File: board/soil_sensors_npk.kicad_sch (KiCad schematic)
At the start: 7 parts, among them J2 Conn_01x04_MountingPin, U6 MAX3485

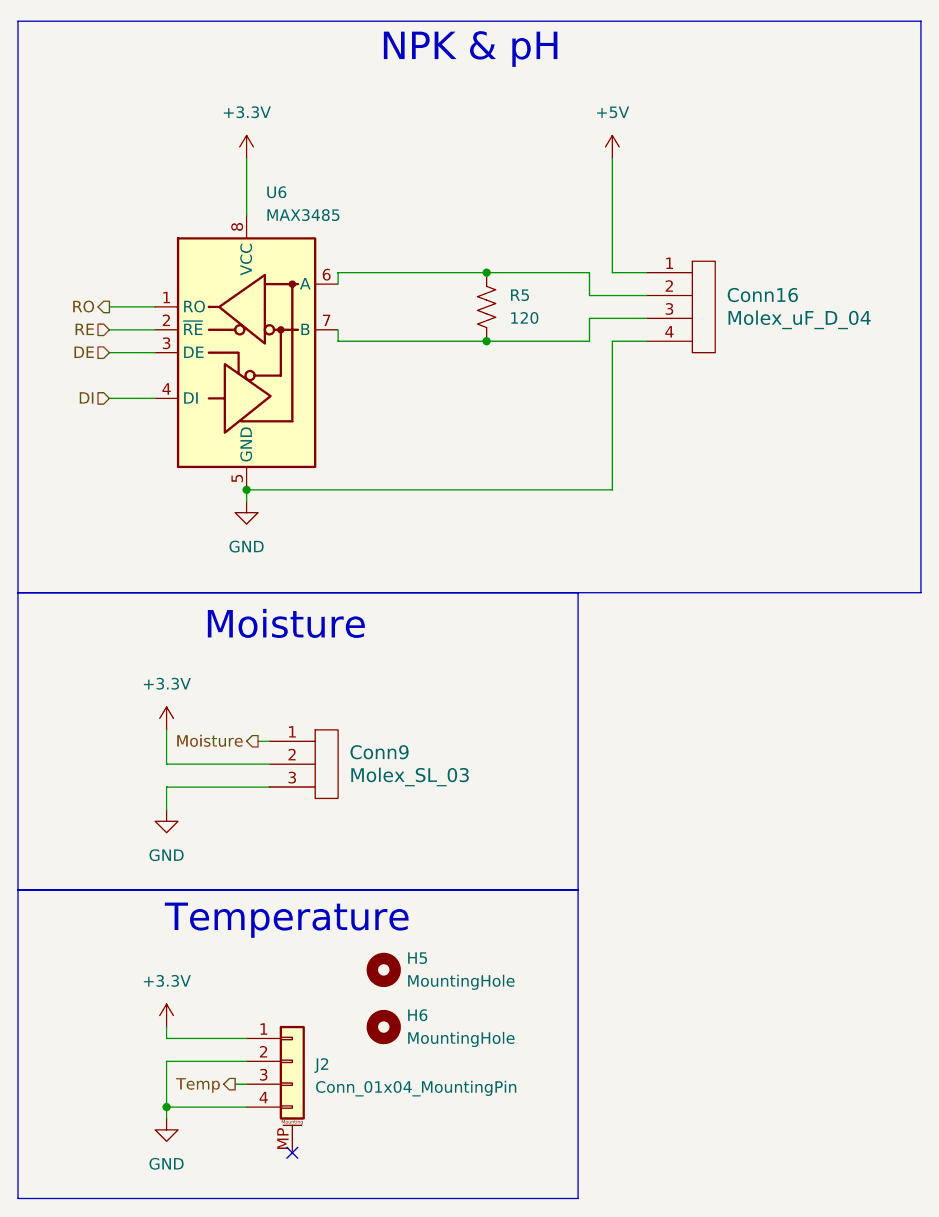
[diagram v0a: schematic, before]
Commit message: Redesigning Layout
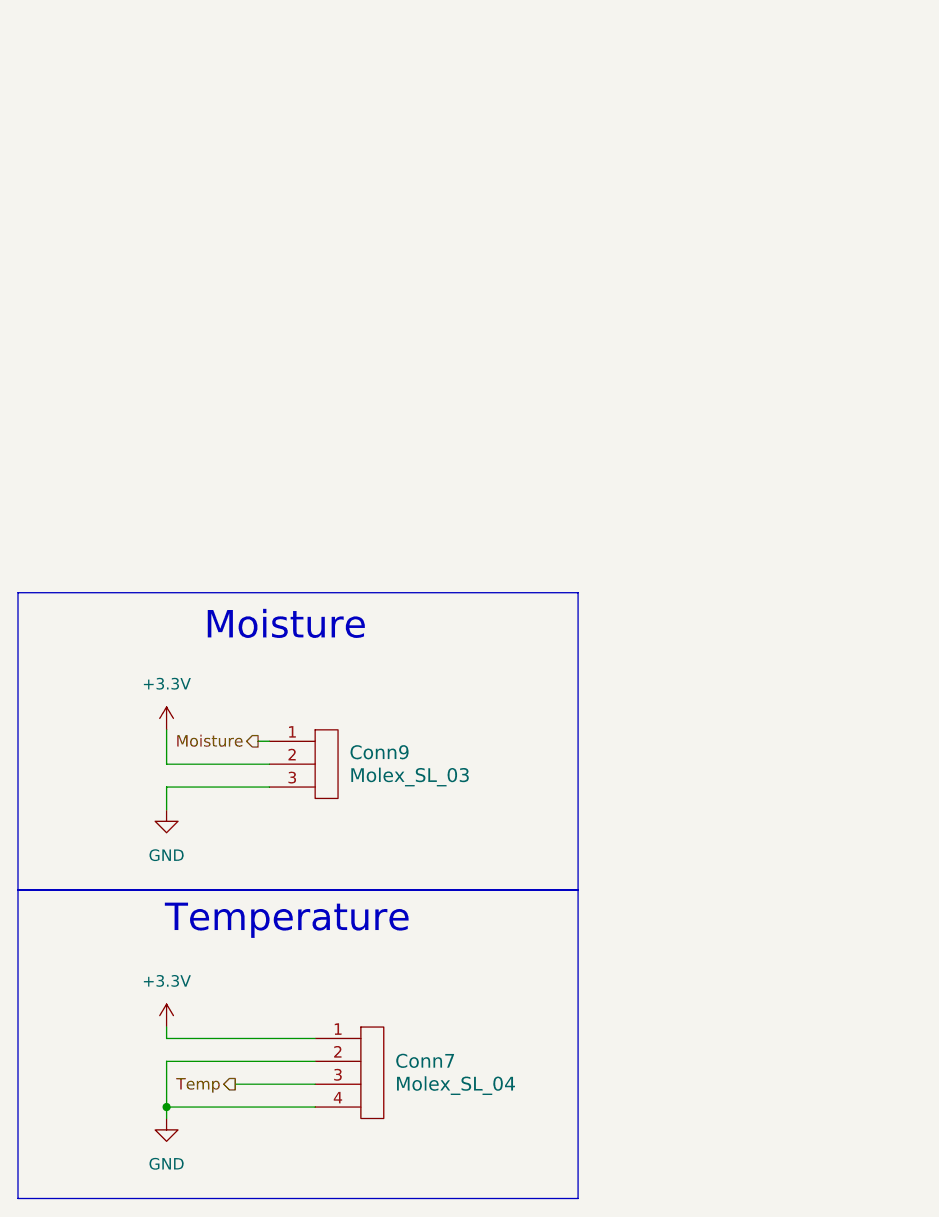
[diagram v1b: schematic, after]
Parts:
- removed Conn16: Molex_uF_D_04, MRDT_Connectors:MOLEX_SL_04_Vertical, symbol MRDT_Connectors:Molex_uF_D_04
- removed H5, H6: MountingHole, MountingHole:MountingHole_2.7mm, symbol Mechanical:MountingHole
- removed J2: Conn_01x04_MountingPin, Connector_PinHeader_2.54mm:PinHeader_1x04_P2.54mm_Vertical, symbol Connector_Generic_MountingPin:Conn_01x04_MountingPin
- removed R5: 120, Resistor_SMD:R_0603_1608Metric_Pad0.98x0.95mm_HandSolder, symbol Device:R_US
- removed U6: MAX3485, Package_SO:SOIC-8_3.9x4.9mm_P1.27mm, symbol Interface_UART:MAX3485
- added Conn7: Molex_SL_04, MRDT_Connectors:MOLEX_SL_04_Vertical, symbol MRDT_Connectors:Molex_SL_04
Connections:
- net +3.3V: now also Conn7.1
- net GND: now also Conn7.2, Conn7.4
- net Temp: now also Conn7.3
- no-connect marks 1 -> 0
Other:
- note removed: "NPK & pH"
